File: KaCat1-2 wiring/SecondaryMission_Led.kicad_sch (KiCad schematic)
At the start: 5 parts, among them U1 LM317L

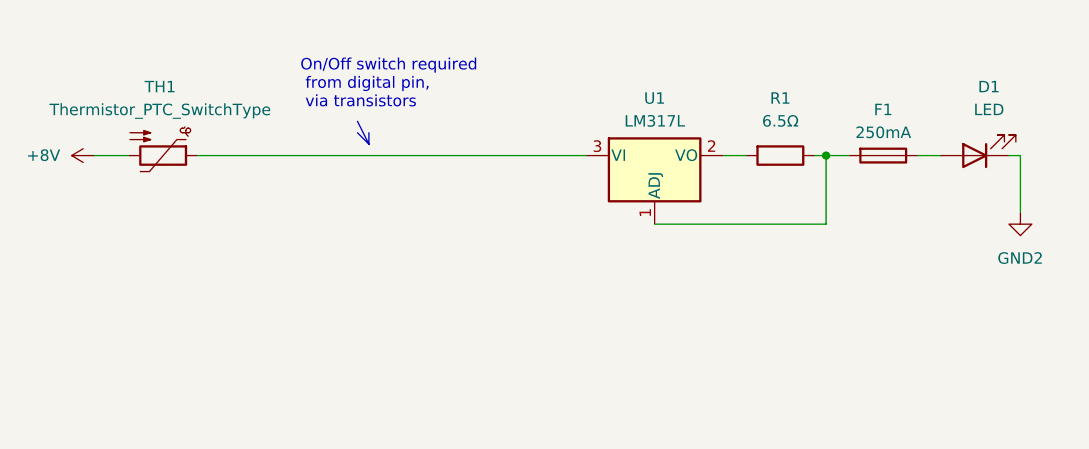
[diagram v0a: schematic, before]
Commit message: Add files via upload
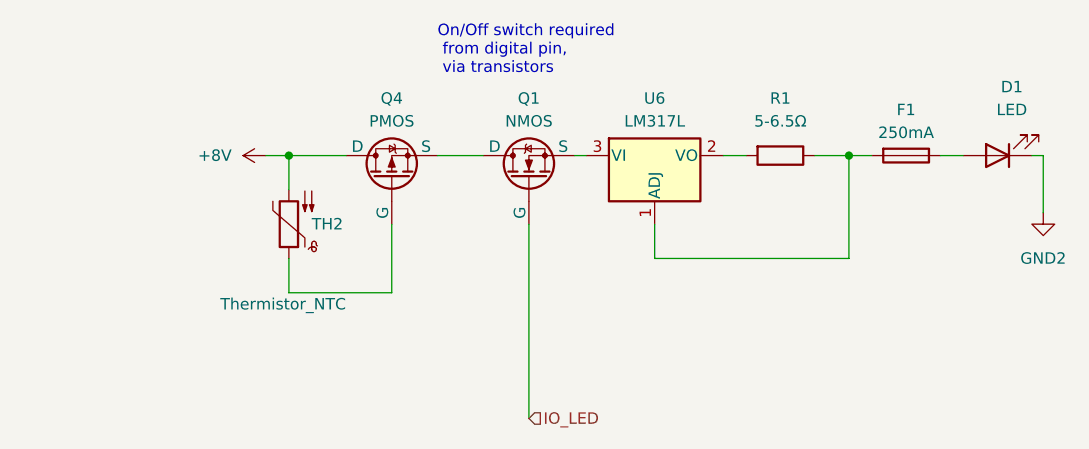
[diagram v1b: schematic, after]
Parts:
- removed TH1: Thermistor_PTC_SwitchType, symbol Device:Thermistor_PTC
- added Q1: NMOS, symbol Simulation_SPICE:NMOS
- added Q4: PMOS, symbol Simulation_SPICE:PMOS
- added TH2: Thermistor_NTC, symbol Device:Thermistor_PTC
- R1: value 6.5Ω -> 5-6.5Ω
- renumbered U1 to U6
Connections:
- net +8V: now also Q4.1 (D), TH2.2
- net at U6.3 (VI): now also Q1.3 (S)
- new net: Q1.1 (D), Q4.3 (S)
- new net: Q4.2 (G), TH2.1
- new net IO_LED: Q1.2 (G)
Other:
- moved on the sheet: D1, F1
